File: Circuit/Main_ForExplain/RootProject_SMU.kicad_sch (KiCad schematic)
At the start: 22 parts, among them J1 Conn_01x04_Pin, J10 Conn_01x03_Socket, J11 Conn_01x03_Pin, J12 Conn_Coaxial, J13 Conn_01x04_Pin, J14 Conn_01x04_Socket, J15 Conn_Coaxial, J16 Conn_Coaxial, J17 Conn_Coaxial, J18 Conn_01x04_Pin, J19 Conn_01x04_Pin, J2 Conn_01x04_Socket, J20 Conn_01x04_Socket, J3 Conn_Coaxial, J4 Conn_Coaxial, J5 Conn_01x04_Pin, J6 Conn_01x04_Socket, J7 MJ-179PH, J8 Conn_01x03_Pin, J9 Conn_01x03_Socket, SW1 SW_SPDT

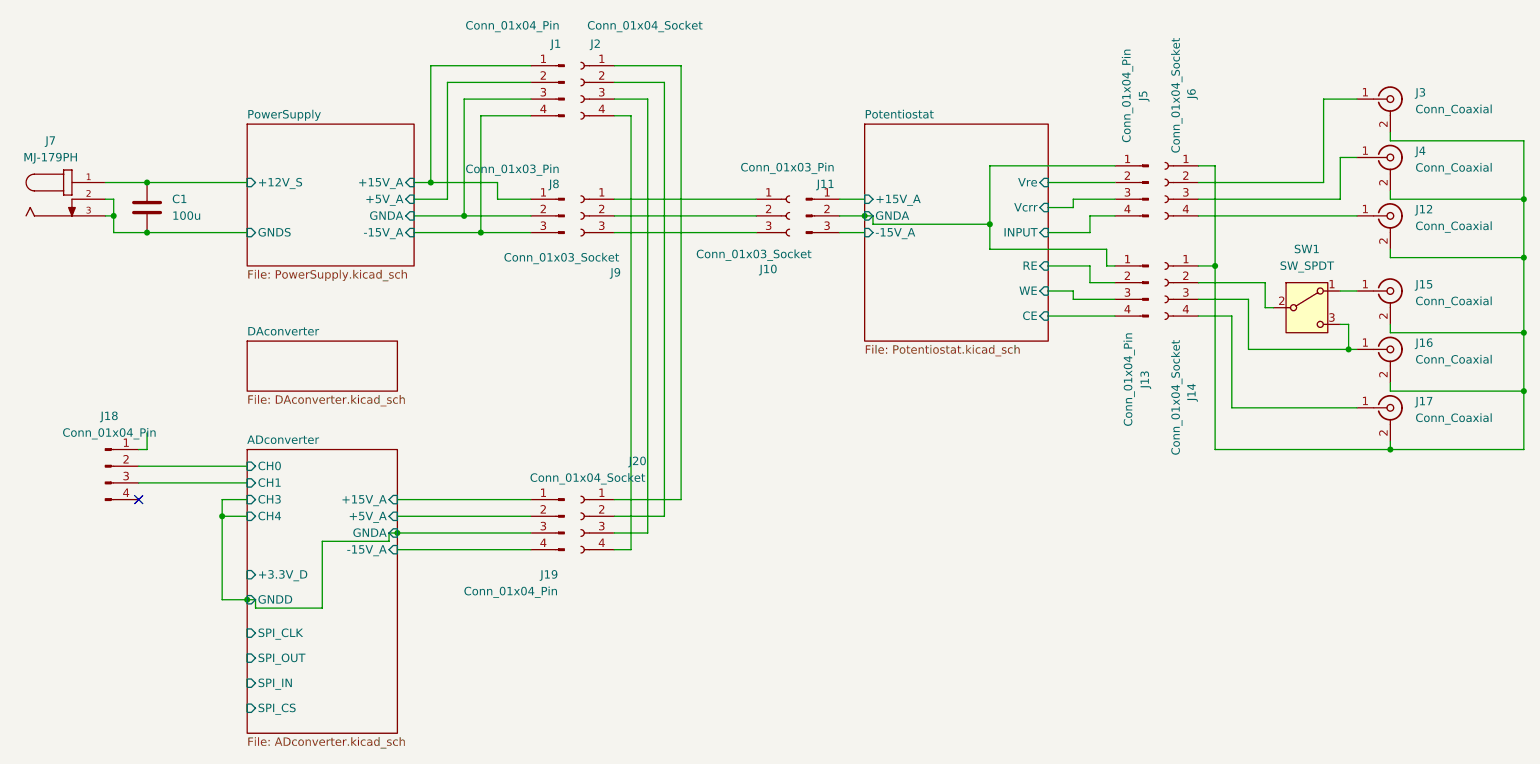
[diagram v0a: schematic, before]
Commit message: 平均化機能を追加
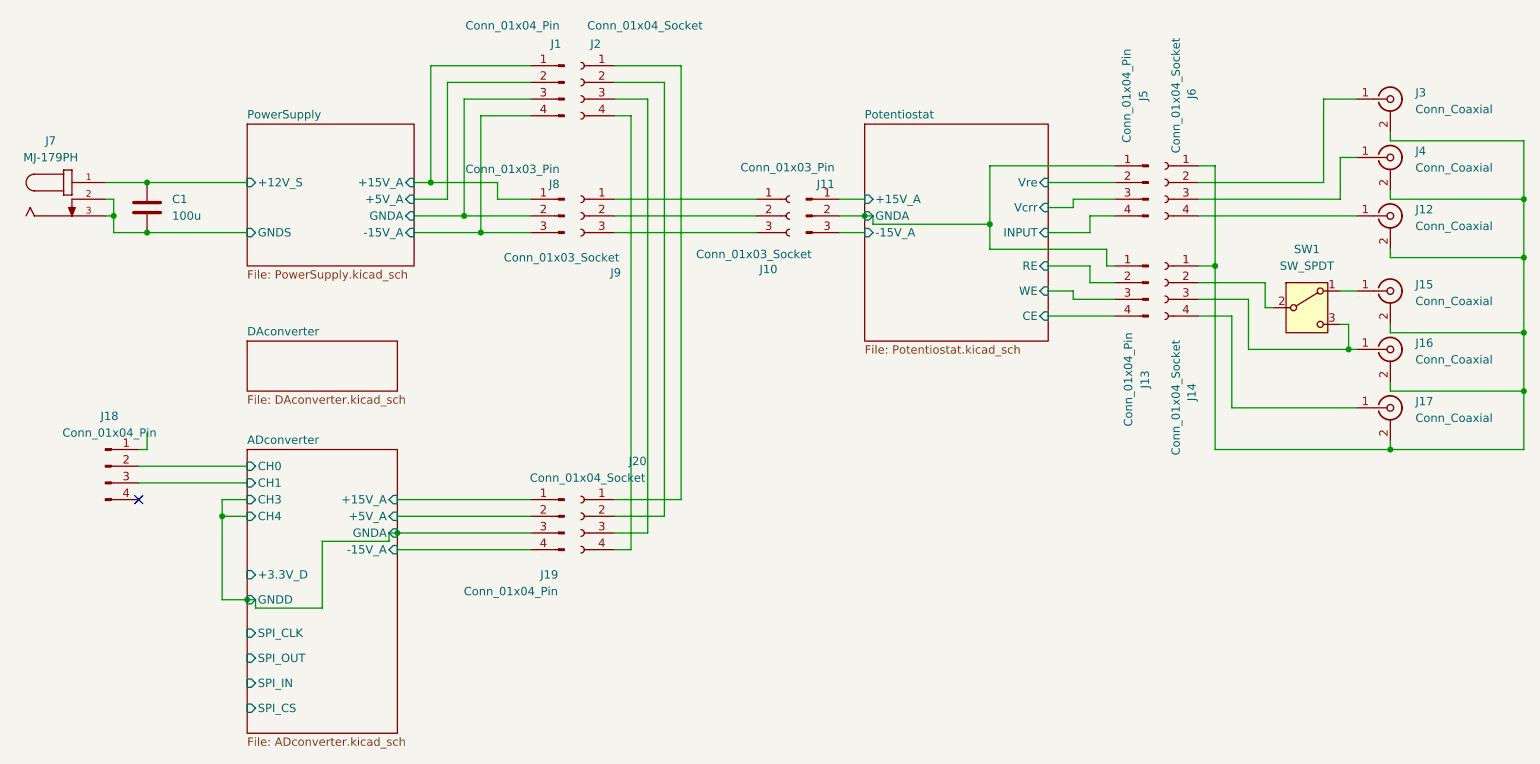
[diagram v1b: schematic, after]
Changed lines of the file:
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@@
 (kicad_sch
-	(version 20231120)
+	(version 20250114)
 	(generator "eeschema")
-	(generator_version "8.0")
+	(generator_version "9.0")
 	(paper "A4")
 	(junction
@@
 		(at 59.69 99.06)
 		(size 22.86 7.62)
+		(exclude_from_sim no)
+		(in_bom yes)
+		(on_board yes)
+		(dnp no)
 		(fields_autoplaced yes)
 		(stroke
@@
 		(at 153.67 66.04)
 		(size 27.94 33.02)
+		(exclude_from_sim no)
+		(in_bom yes)
+		(on_board yes)
+		(dnp no)
 		(fields_autoplaced yes)
 		(stroke
@@
 		(at 59.69 115.57)
 		(size 22.86 43.18)
+		(exclude_from_sim no)
+		(in_bom yes)
+		(on_board yes)
+		(dnp no)
 		(fields_autoplaced yes)
 		(stroke
@@
 		(at 59.69 66.04)
 		(size 25.4 21.59)
+		(exclude_from_sim no)
+		(in_bom yes)
+		(on_board yes)
+		(dnp no)
 		(fields_autoplaced yes)
 		(stroke
@@
 		)
 	)
+	(embedded_fonts no)
 )
